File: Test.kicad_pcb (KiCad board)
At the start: 2 copper layers, 128 x 80.5 mm, 14 parts, among them P1 USB_C_Receptacle_USB2.0, SW1 SW_Push, U1 ATmega328P-P, U2 CH340N, U3 AMS1117, Y1 Crystal

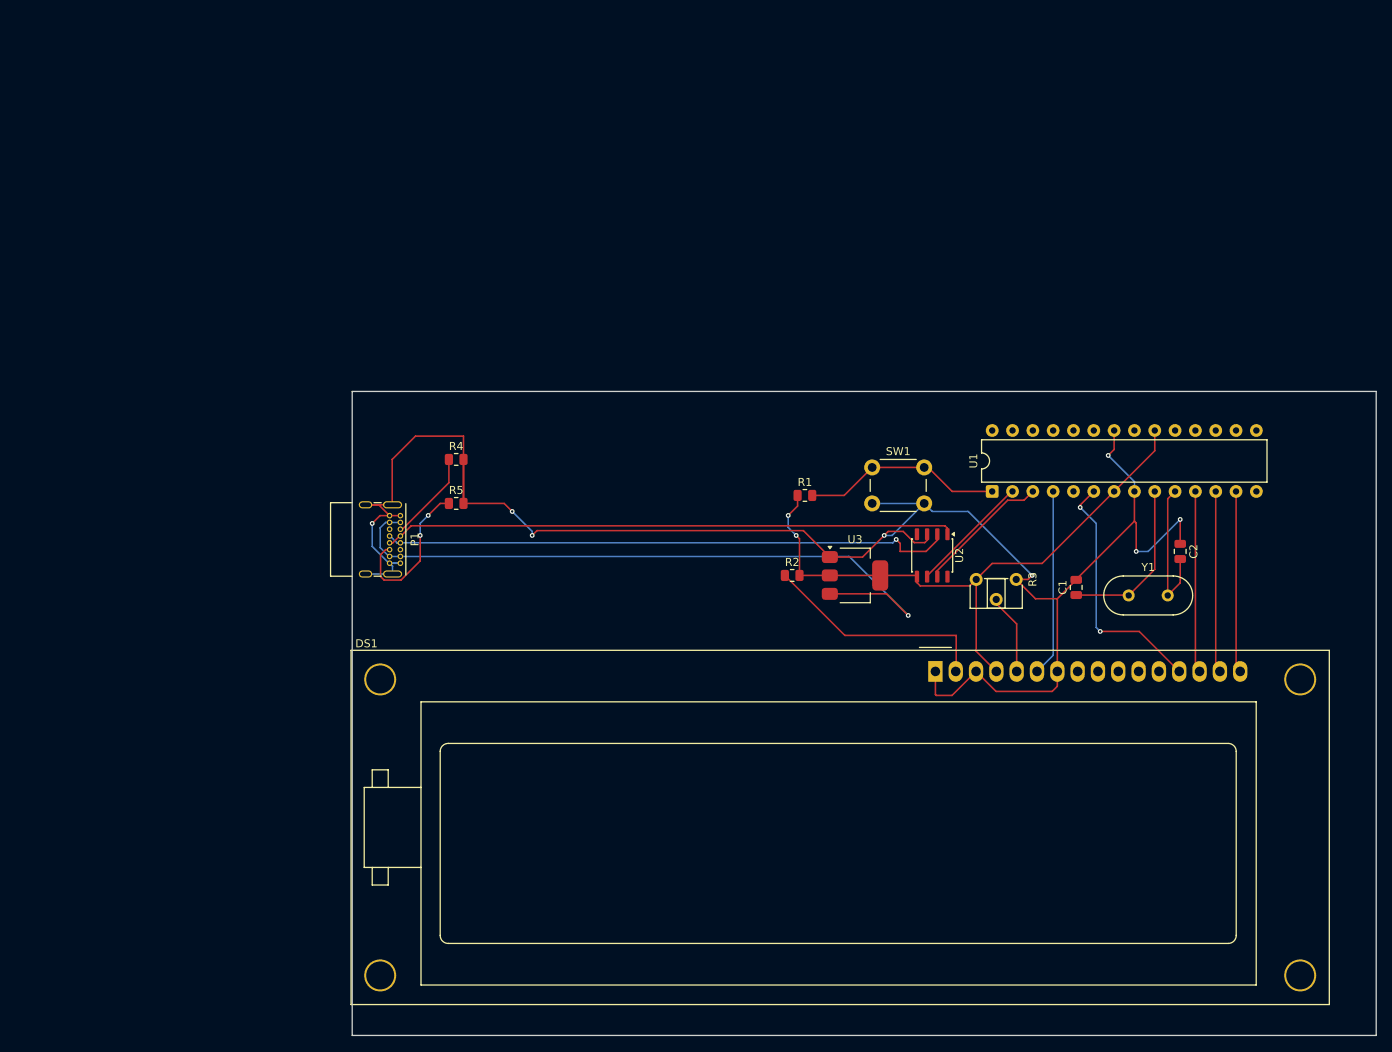
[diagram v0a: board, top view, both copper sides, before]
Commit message: Update Test.kicad_pcb
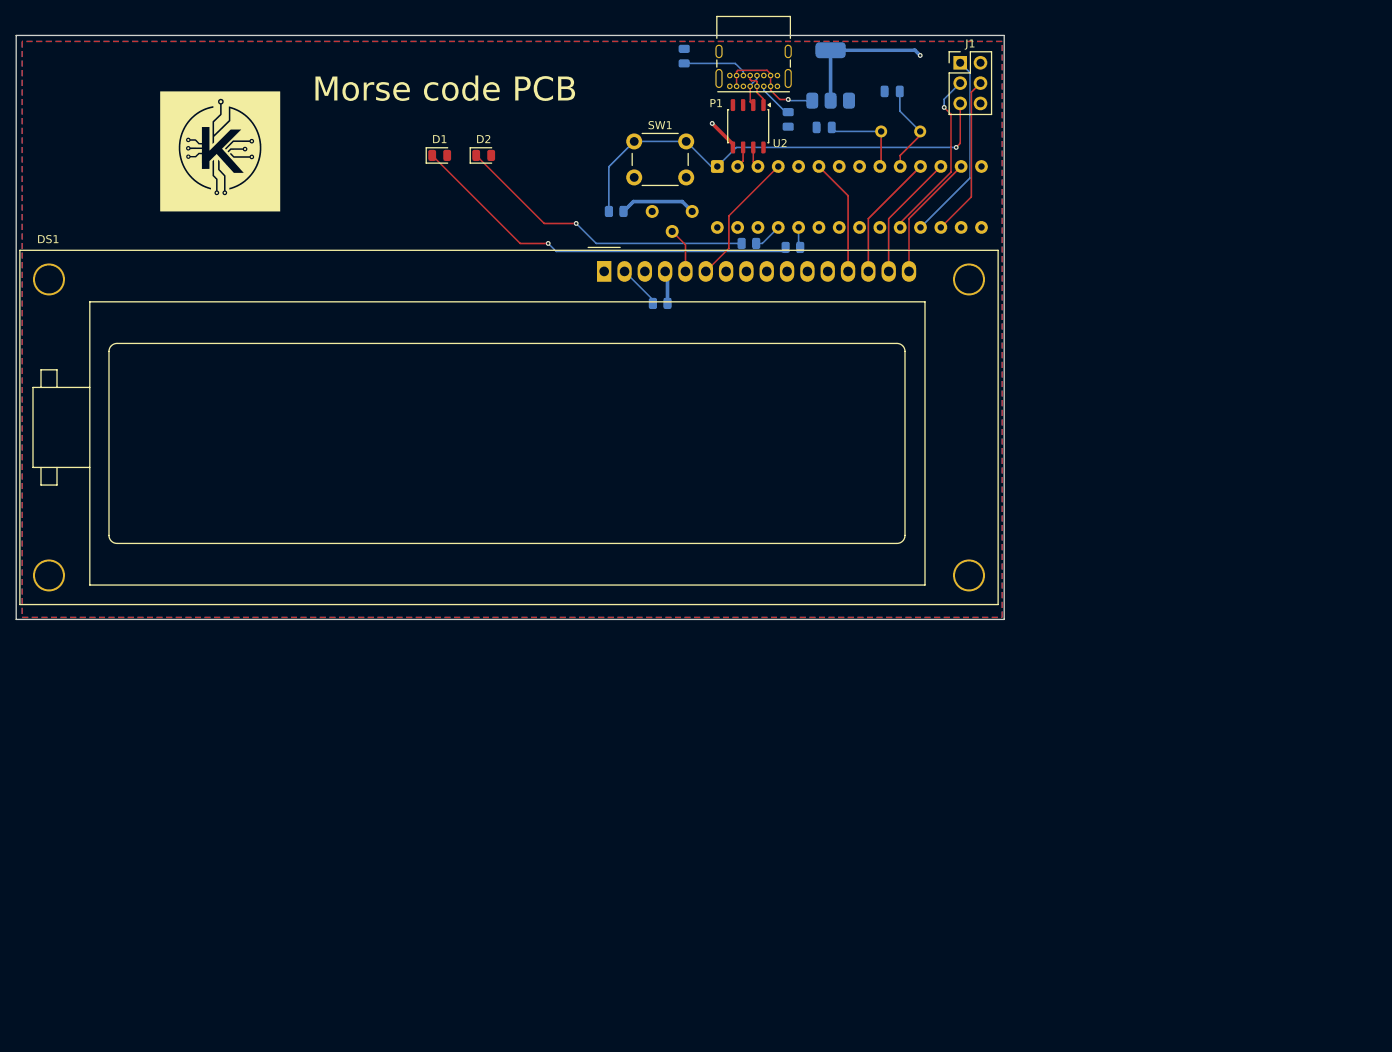
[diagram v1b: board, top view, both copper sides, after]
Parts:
- added D1: LED1, LED_SMD:LED_0805_2012Metric, F.Cu at (127.4, 81.5)
- added D2: LED2, LED_SMD:LED_0805_2012Metric, F.Cu at (132.9, 81.5)
- added G***: LOGO, LOGO, F.Cu at (100.0, 81.0)
- added J1: AVR-ISP-6, Connector_PinHeader_2.54mm:PinHeader_2x03_P2.54mm_Vertical, F.Cu at (192.5, 69.9)
- added R6: 220, Resistor_SMD:R_0805_2012Metric, B.Cu at (171.6, 93.0)
- added R7: 220, Resistor_SMD:R_0805_2012Metric, B.Cu at (166.1, 92.5)
- C1, C2, R1, R2, R3, R4, R5, U1, U3, Y1: moved to B.Cu
- moved P1 71.4 mm to (169.7, 72.9), turned to 180 degrees
- moved C2 67.8 mm to (184.0, 73.5), turned to 0 degrees
- moved Y1 65.7 mm to (182.6, 78.5)
- moved C1 65.6 mm to (175.5, 78.0), turned to 180 degrees
- moved DS1 64.9 mm to (148.0, 96.0)
- moved R3 64.7 mm to (154.0, 88.5)
- moved R5 62.8 mm to (158.0, 69.1), turned to 90 degrees
- moved U3 62.6 mm to (176.3, 71.5), turned to 90 degrees
- moved R4 59.4 mm to (171.0, 77.0), turned to -90 degrees
- moved U2 58.4 mm to (166.0, 77.8)
- moved U1 53.2 mm to (162.1, 82.9), turned to -90 degrees
- moved SW1 50.5 mm to (151.8, 79.8)
- moved R1 42.6 mm to (149.5, 88.5), turned to 180 degrees
- moved R2 37.8 mm to (155.0, 100.0)
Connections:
- net Net-(U1-~{RESET}/PC6) renamed RST
- U1 pad 17: unconnected-(U1-PB3-Pad17) -> Mosi
- U1 pad 18: unconnected-(U1-PB4-Pad18) -> Miso
- U1 pad 19: unconnected-(U1-PB5-Pad19) -> SCK
- U1 pad 24: unconnected-(U1-PC1-Pad24) -> PC1
- U1 pad 25: unconnected-(U1-PC2-Pad25) -> PC2
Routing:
- net GND: track 229.6 -> 0.00 mm, vias 8 -> 0
- net Net-(U3-VI): track 85.7 -> 14.1 mm
- net USB_C D-: track 71.5 -> 4.20 mm, vias 1 -> 0
- net USB_C D+: track 71.5 -> 4.72 mm
- net Net-(D1-K): track 0.00 -> 49.4 mm, vias 0 -> 1
- net +5V: track 78.5 -> 35.6 mm
- net Net-(D2-K): track 0.00 -> 37.7 mm, vias 0 -> 1
- net RST: track 25.2 -> 58.3 mm, vias 0 -> 1
- net Miso: track 0.00 -> 23.6 mm
- net Net-(DS1-LEDA): track 29.0 -> 5.47 mm
- net SCK: track 0.00 -> 21.9 mm, vias 0 -> 1
- net Mosi: track 0.00 -> 20.1 mm
- net Net-(DS1-DB4): track 31.2 -> 14.6 mm, vias 2 -> 0
- net CH340N_RX: track 16.8 -> 2.62 mm
- net CH340N_TX: track 15.1 -> 2.66 mm
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- added copper zone on In1.Cu, net +5V
- added copper zone on B.Cu, net GND
- added copper zone on F.Cu, net GND
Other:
- board size 128 x 80.5 mm -> 123.5 x 73 mm
- copper layers 2 -> 4
- board text added: "Morse code PCB"
